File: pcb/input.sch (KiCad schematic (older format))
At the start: 24 parts, among them J4 CONN_01X16, U1 MCP23017, U2 LTV-847, U3 LTV-847, U4 LTV-847, U5 LTV-847

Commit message: Updating PCB
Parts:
- removed C?: 0.1uF, symbol C
- removed C?: 22uF, symbol CP
- removed J4: CONN_01X16, symbol CONN_01X16
- removed R1, R10, R11, R12, R13, R14, R15, R16, R2, R3, R4, R5, R6, R7, R8, R9: 470, symbol R
- removed U1: MCP23017, symbol MCP23017
- removed U2, U3, U4, U5: LTV-847, Housings_DIP:DIP-16_W7.62mm, symbol LTV-847
- added C3: 0.1uF, Capacitor_THT:C_Disc_D5.0mm_W2.5mm_P2.50mm, symbol Device:C
- added J10, J9: Screw_Terminal_01x08, TerminalBlock_TE-Connectivity:TerminalBlock_TE_282834-8_1x08_P2.54mm_Horizontal, symbol Connector:Screw_Terminal_01x08
- added U2: MCP23017-E_SP, Package_DIP:DIP-28_W7.62mm, symbol dk_Interface-I-O-Expanders:MCP23017-E_SP
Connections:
- net labels added: Pin0, Pin1, Pin10, Pin11, Pin12, Pin13, Pin14, Pin15, Pin2, Pin3, Pin4, Pin5, Pin6, Pin7, Pin8, Pin9, ~RESET
- net labels removed: GNDD, GPA0, GPA1, GPA2, GPA3, GPA4, GPA5, GPA6, GPA7, GPA[0..3], GPA[0..7], GPA[4..7], GPB0, GPB1, GPB2, GPB3, GPB4, GPB5, GPB6, GPB7, GPB[0..3], GPB[0..7], GPB[4..7], IN[0..15], IN[0..3], IN[0..7], IN[12..15], IN[4..7], IN[8..11], IN[8..15], RESET
- wire segments 126 -> 78

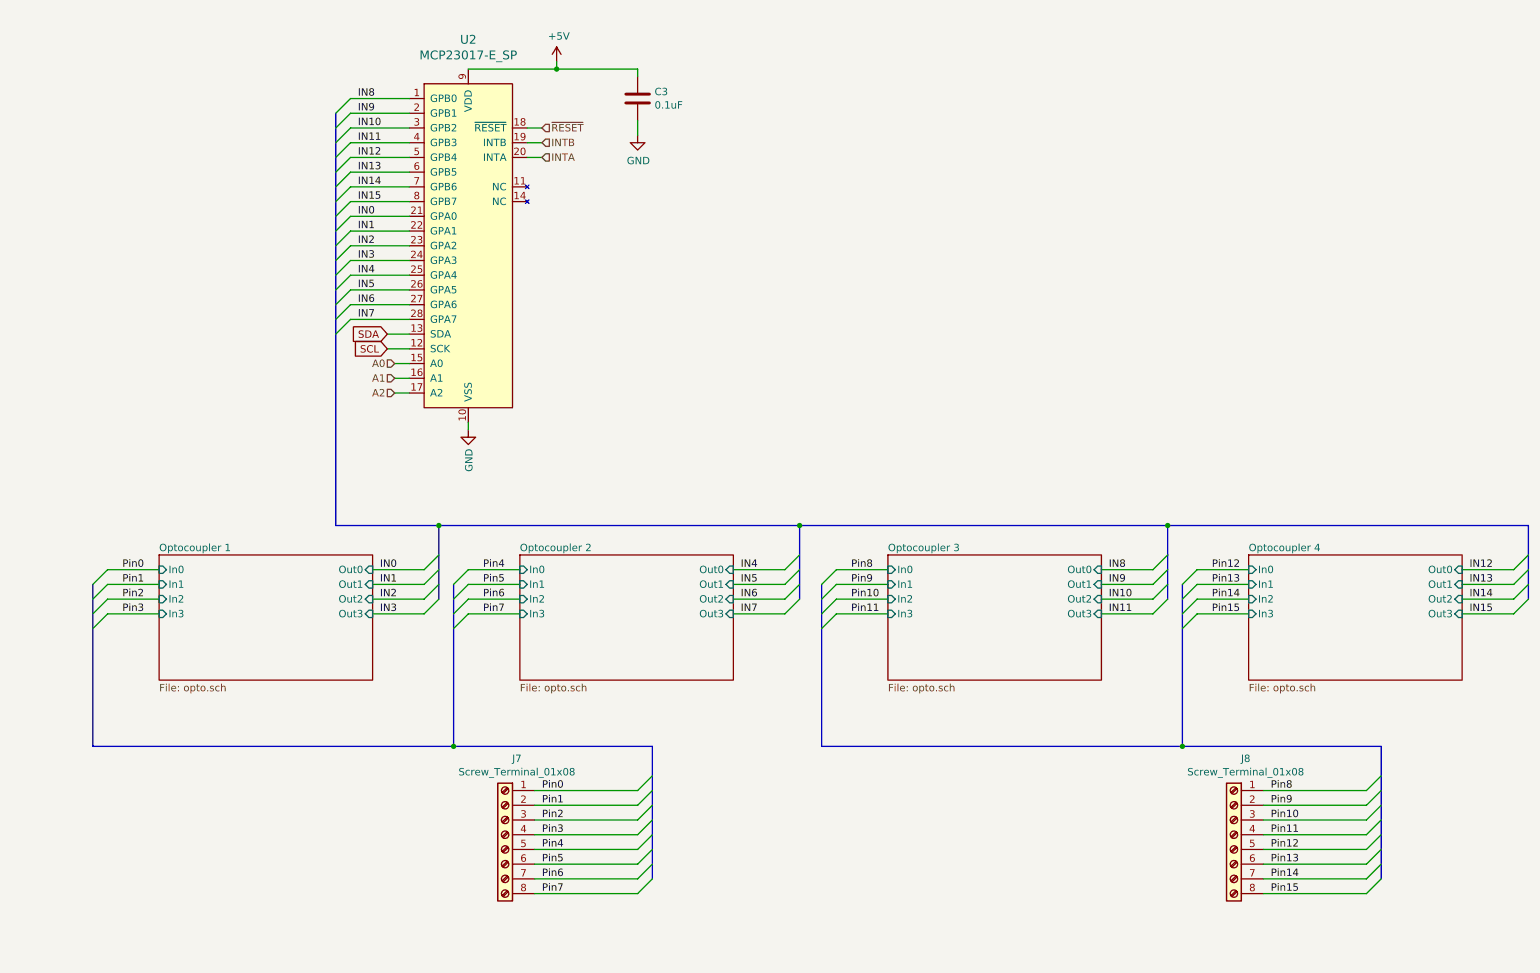
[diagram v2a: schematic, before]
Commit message: latest
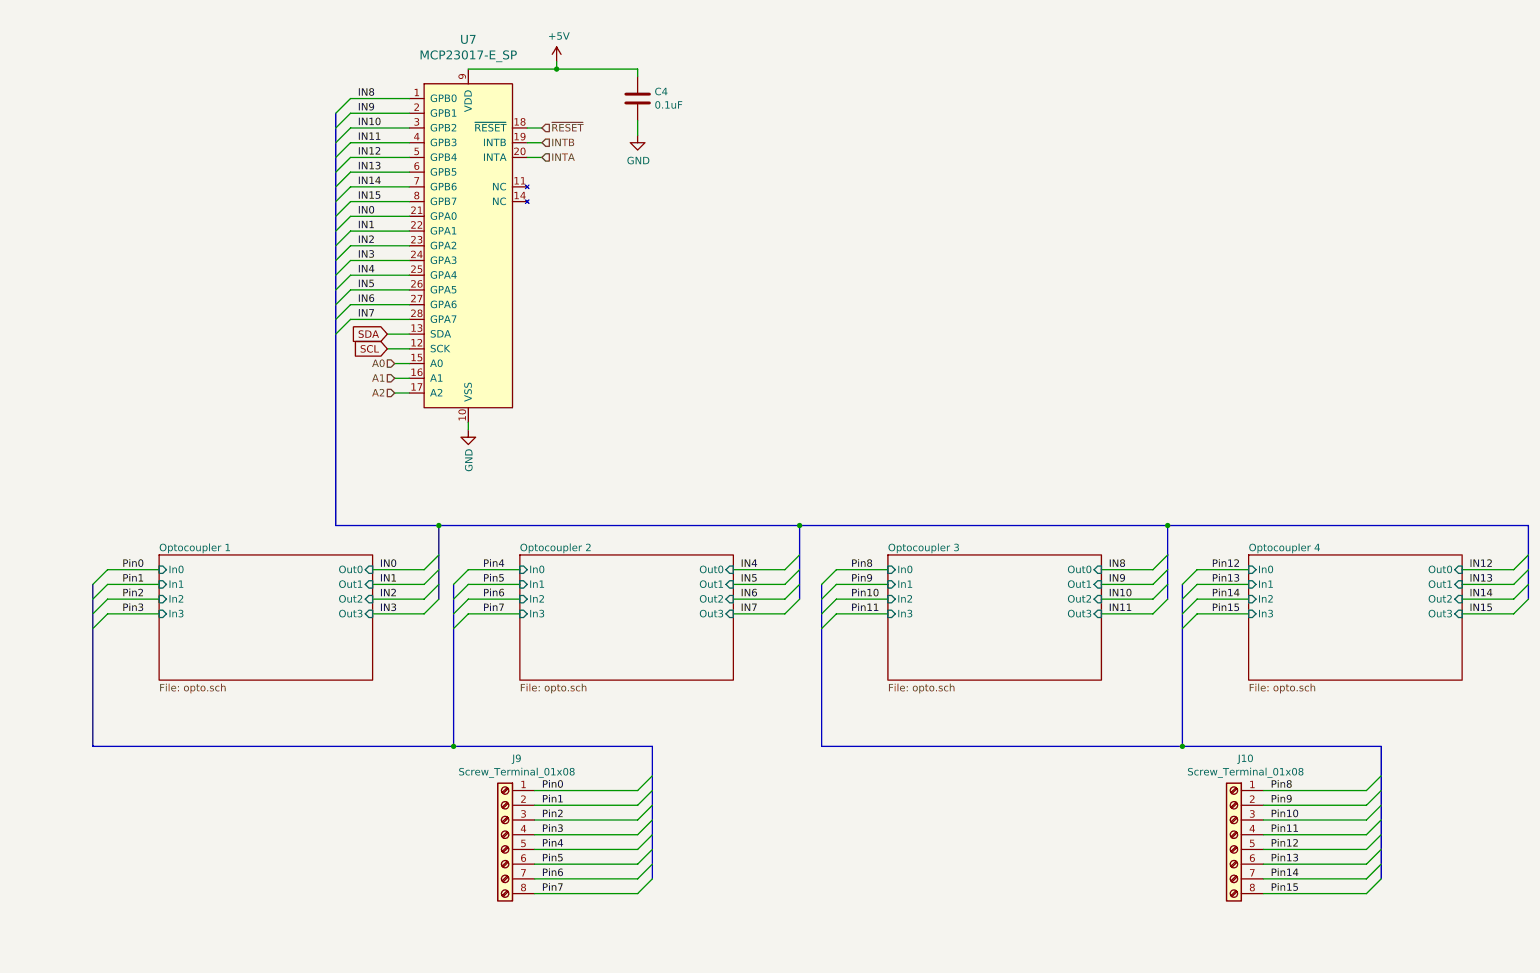
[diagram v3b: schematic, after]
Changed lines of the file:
@@
 AR Path="/5C211542/5C211768" Ref="U2"  Part="1"
 AR Path="/5C211551/5C211768" Ref="U7"  Part="1"
-F 0 "U2" H 3850 2600 60  0000 C CNN
+F 0 "U7" H 3850 2600 60  0000 C CNN
 F 1 "MCP23017-E_SP" H 3850 2494 60  0000 C CNN
 F 2 "Package_DIP:DIP-28_W7.62mm" H 3950 1800 60  0001 L CNN
@@
 AR Path="/5C211542/5C211A11" Ref="#PWR025"  Part="1"
 AR Path="/5C211551/5C211A11" Ref="#PWR036"  Part="1"
-F 0 "#PWR025" H 4450 600 50  0001 C CNN
+F 0 "#PWR036" H 4450 600 50  0001 C CNN
 F 1 "+5V" H 4465 923 50  0000 C CNN
 F 2 "" H 4450 750 50  0001 C CNN
@@
 AR Path="/5C211542/5C2127BA" Ref="#PWR024"  Part="1"
 AR Path="/5C211551/5C2127BA" Ref="#PWR035"  Part="1"
-F 0 "#PWR024" H 3850 3000 50  0001 C CNN
+F 0 "#PWR035" H 3850 3000 50  0001 C CNN
 F 1 "GND" V 3855 3122 50  0000 R CNN
 F 2 "" H 3850 3250 50  0001 C CNN
@@
 AR Path="/5C211542/5C2C6D1A" Ref="C3"  Part="1"
 AR Path="/5C211551/5C2C6D1A" Ref="C4"  Part="1"
-F 0 "C3" H 5115 1046 50  0000 L CNN
+F 0 "C4" H 5115 1046 50  0000 L CNN
 F 1 "0.1uF" H 5115 955 50  0000 L CNN
 F 2 "Capacitor_THT:C_Disc_D5.0mm_W2.5mm_P2.50mm" H 5038 850 50  0001 C CNN
@@
 AR Path="/5C211542/5C2C6D8B" Ref="#PWR026"  Part="1"
 AR Path="/5C211551/5C2C6D8B" Ref="#PWR037"  Part="1"
-F 0 "#PWR026" H 5000 1000 50  0001 C CNN
+F 0 "#PWR037" H 5000 1000 50  0001 C CNN
 F 1 "GND" H 5005 1077 50  0000 C CNN
 F 2 "" H 5000 1250 50  0001 C CNN
@@
 AR Path="/5C211551/5C2B8202" Ref="J9"  Part="1"
 AR Path="/5C211542/5C2B8202" Ref="J7"  Part="1"
-F 0 "J7" H 4020 6517 50  0000 C CNN
+F 0 "J9" H 4020 6517 50  0000 C CNN
 F 1 "Screw_Terminal_01x08" H 4020 6426 50  0000 C CNN
 F 2 "TerminalBlock_TE-Connectivity:TerminalBlock_TE_282834-8_1x08_P2.54mm_Horizontal" H 4100 6000 50  0001 C CNN
@@
 AR Path="/5C211551/5C2BD2C4" Ref="J10"  Part="1"
 AR Path="/5C211542/5C2BD2C4" Ref="J8"  Part="1"
-F 0 "J8" H 8970 6517 50  0000 C CNN
+F 0 "J10" H 8970 6517 50  0000 C CNN
 F 1 "Screw_Terminal_01x08" H 8970 6426 50  0000 C CNN
 F 2 "TerminalBlock_TE-Connectivity:TerminalBlock_TE_282834-8_1x08_P2.54mm_Horizontal" H 9050 6000 50  0001 C CNN
